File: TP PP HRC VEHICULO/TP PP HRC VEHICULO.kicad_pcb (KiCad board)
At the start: 2 copper layers, 100 x 100 mm, 56 parts, among them J10 Conn_01x04_Pin, J2 Conn_01x01_Pin, J3 Conn_01x01_Pin, J5vgnd1 Screw_Terminal_01x02, J6 Conn_01x04_Pin, J7 USB_B, J9 Conn_01x04_Pin, K1 Relay_SPDT, K2 Relay_SPDT, SW1 SW_Push, SW2 SW_Push, U1 ESP32-Devkit-V1, U2 LM317L_TO92

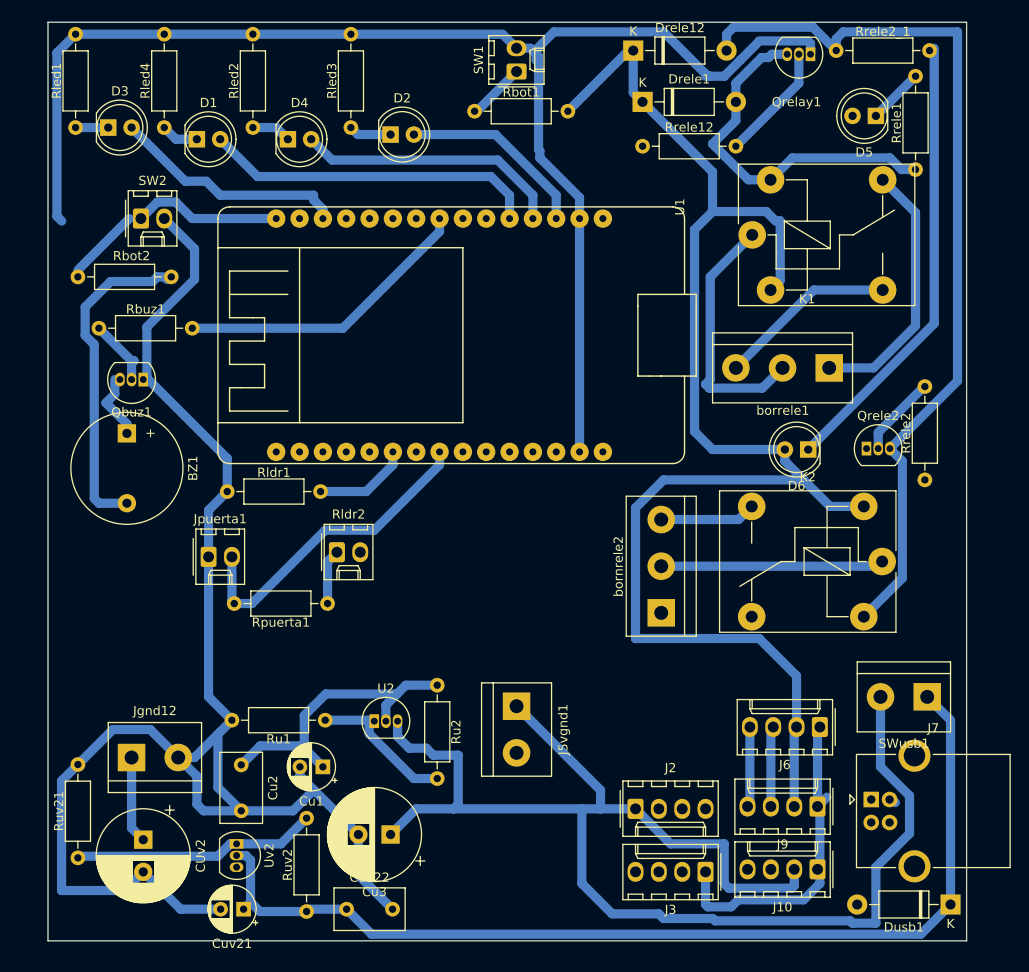
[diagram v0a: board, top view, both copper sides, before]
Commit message: si
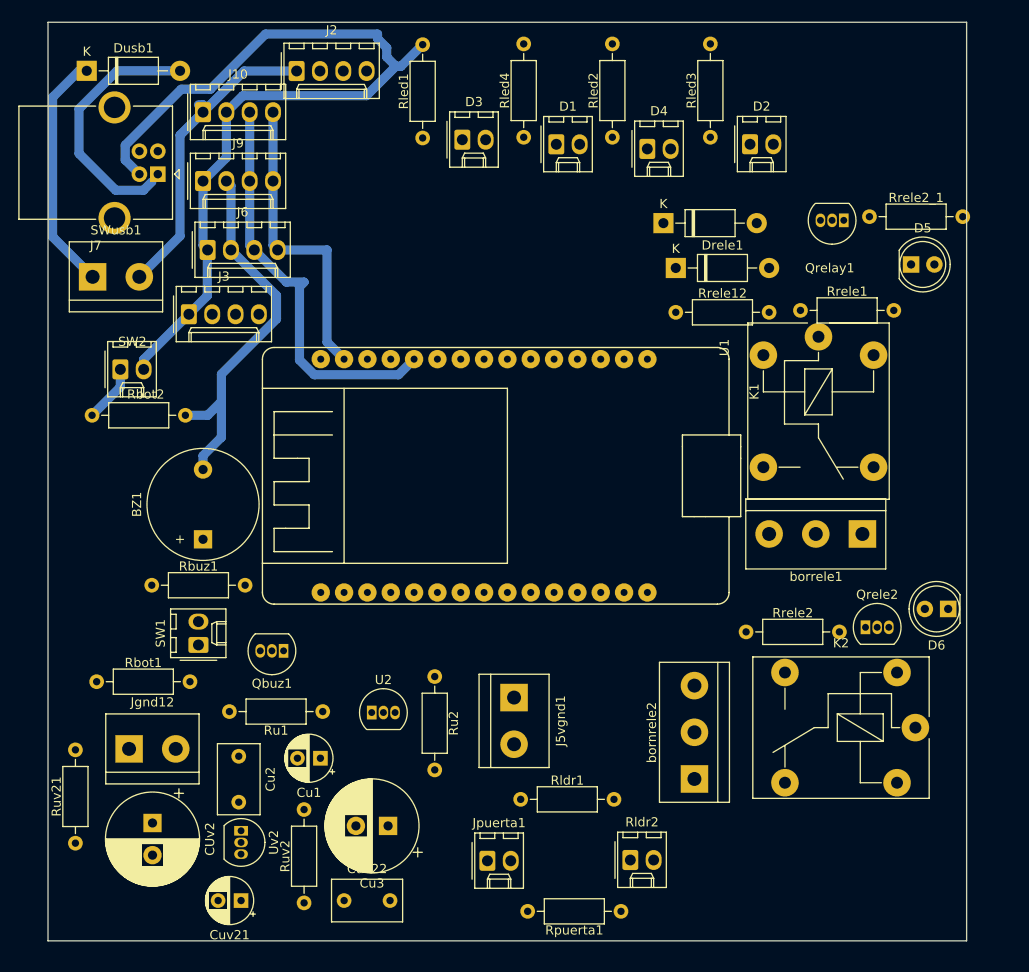
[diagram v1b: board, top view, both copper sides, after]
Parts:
- D1, D2, D3, D4: footprint LED_THT:LED_D5.0mm -> Connector_Molex:Molex_KK-254_AE-6410-02A_1x02_P2.54mm_Vertical
- moved Dusb1 130.7 mm to (120.3, 68.5), turned to 0 degrees
- moved J10 106.2 mm to (133.0, 73.0), turned to 0 degrees
- moved J7 103.3 mm to (128.1, 79.8), turned to 180 degrees
- moved SWusb1 101.7 mm to (121.0, 90.9), turned to 0 degrees
- moved J9 95.5 mm to (133.0, 80.5), turned to 0 degrees
- moved J2 88.4 mm to (143.2, 68.5)
- moved J6 84.5 mm to (133.5, 88.0), turned to 0 degrees
- moved J3 82.8 mm to (131.5, 95.0), turned to 0 degrees
- moved Rbot1 74.5 mm to (121.4, 135.0)
- moved SW1 71.4 mm to (132.5, 131.0)
- moved Rldr1 46.3 mm to (167.6, 147.8)
- moved Rpuerta1 46.3 mm to (178.5, 160.0)
- moved Rldr2 46.3 mm to (179.5, 154.4)
- moved Jpuerta1 44.9 mm to (164.0, 154.5)
- moved D2 39.1 mm to (192.5, 76.5)
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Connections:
- J10 pad 1: GND -> +5V
- J10 pad 2: +5V -> GND
- U1 pad 11: RELE_B -> unconnected-(U1-IO35-Pad11)
- U1 pad 12: RELE_A -> unconnected-(U1-IO34-Pad12)
- U1 pad 13: unconnected-(U1-IO39-Pad13) -> BUZZER
- U1 pad 14: unconnected-(U1-IO36-Pad14) -> PUERTA
- U1 pad 18: LED-A1 -> unconnected-(U1-IO1-Pad18)
- U1 pad 22: unconnected-(U1-IO18-Pad22) -> RELE_A
- U1 pad 23: BUZZER -> RELE_B
- U1 pad 24: unconnected-(U1-IO17-Pad24) -> LED-A1
- U1 pad 25: unconnected-(U1-IO16-Pad25) -> LED-B2
- U1 pad 26: LED-B2 -> LED-B1
- U1 pad 27: LED-B1 -> LED-A2
- U1 pad 28: LED-A2 -> BOT_B
- U1 pad 8: PUERTA -> unconnected-(U1-IO25-Pad8)
- U1 pad 9: BOT_B -> unconnected-(U1-IO33-Pad9)
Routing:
- net GND: track 359.8 -> 97.4 mm
- net +3.3V: track 203.7 -> 41.5 mm
- net +5V: track 152.6 -> 34.1 mm
- net Net-(Drele12-A): track 98.9 -> 0.00 mm
- net 5V PREVIO AL SWITCH: track 110.7 -> 26.3 mm
- net Net-(D6-K): track 49.4 -> 0.00 mm
- net Net-(Drele1-A): track 39.2 -> 0.00 mm
- net LED-B2: track 36.6 -> 0.00 mm
- net SDA: track 8.76 -> 44.6 mm
- net PUERTA: track 35.2 -> 0.00 mm
- net +3V3: track 33.5 -> 0.00 mm
- net BUZZER: track 32.7 -> 0.00 mm
- net LED-B1: track 29.2 -> 0.00 mm
- net Net-(borrele1-Pin_1): track 28.7 -> 0.00 mm
- net Net-(borrele1-Pin_2): track 27.8 -> 0.00 mm
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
